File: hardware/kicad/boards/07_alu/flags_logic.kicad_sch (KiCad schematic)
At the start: 10 parts, among them U36 74HC86, U37 74LS08, U38 74LS540, U39 74LS377, U40 74LS377

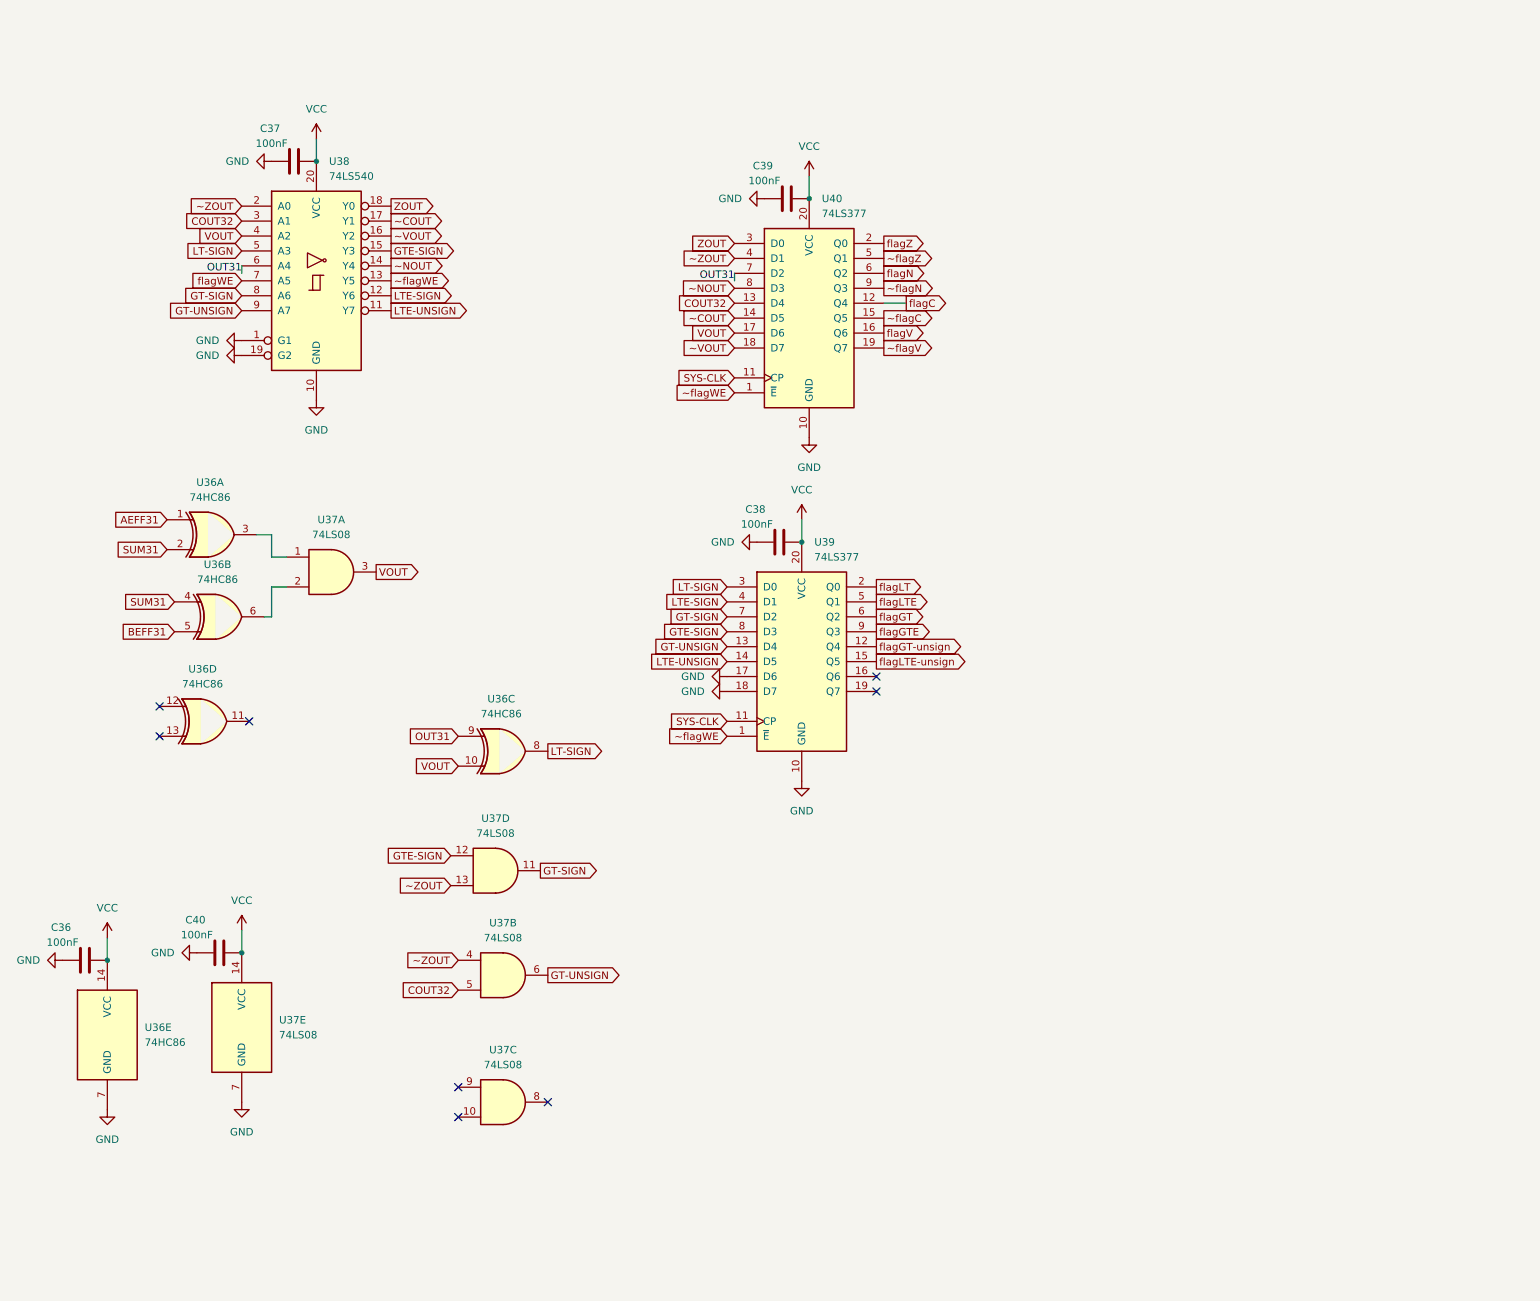
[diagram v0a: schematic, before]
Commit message: checkpoint: most recent 16b cell: ~120mm by 120mm
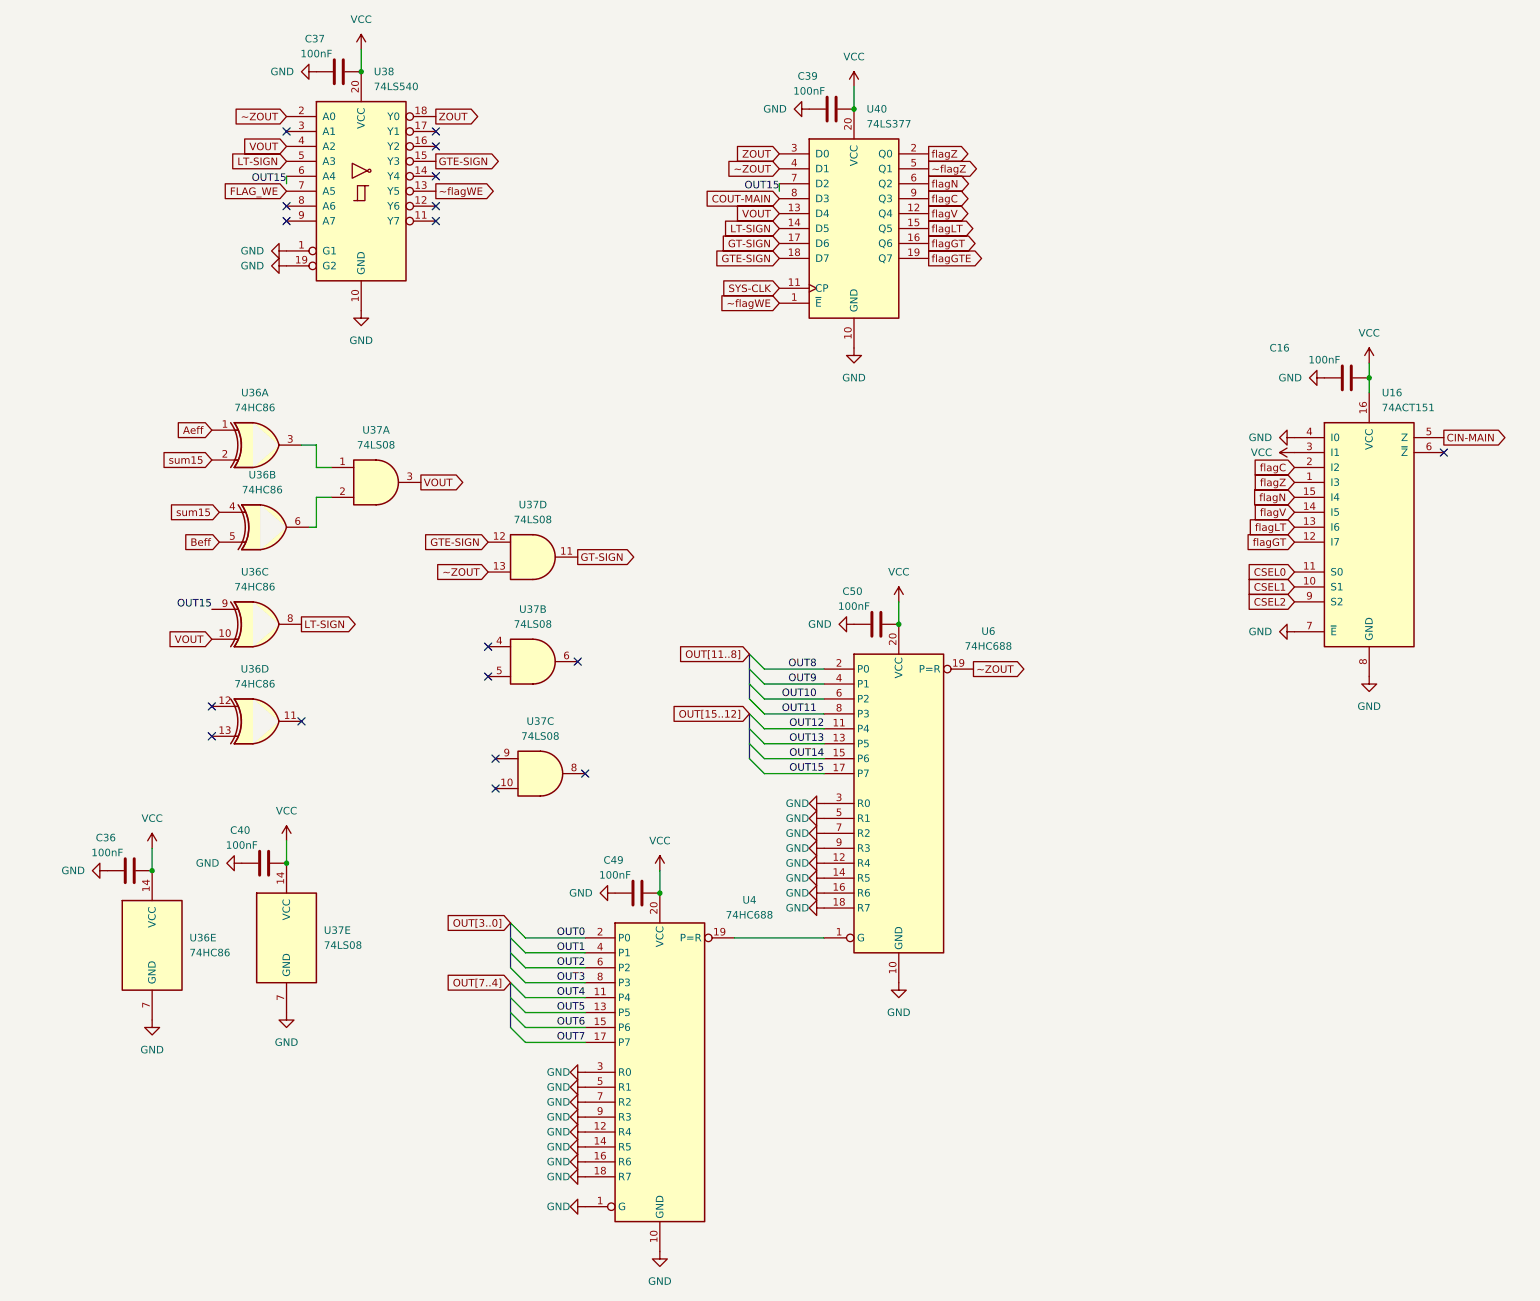
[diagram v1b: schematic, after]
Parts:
- removed C38: 100nF, Capacitor_SMD:C_0603_1608Metric, symbol Device:C
- removed U39: 74LS377, Package_SO:SOIC-20W_7.5x12.8mm_P1.27mm, symbol 74xx:74LS377
- added C16, C49, C50: 100nF, Capacitor_SMD:C_0603_1608Metric, symbol Device:C
- added U16: 74ACT151, Package_SO:SOIC-16_3.9x9.9mm_P1.27mm, symbol 74xx:74LS151
- added U4, U6: 74HC688, Package_SO:SOIC-20W_7.5x12.8mm_P1.27mm, symbol 74xx:74HC688
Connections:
- net ~flagC is gone; now on net flagLT: U40.15 (Q5)
- net ~flagN is gone; now on net flagC: U40.9 (Q3)
- net ~flagV is gone; now on net flagGTE: U40.19 (Q7)
- net GND: now also C16.1, C49.1, C50.1, U16.4 (I0), U16.7 (~{E}), U16.8 (GND), U4.1 (G), U4.10 (GND), U4.12 (R4), U4.14 (R5), U4.16 (R6), U4.18 (R7), U4.3 (R0), U4.5 (R1), U4.7 (R2), U4.9 (R3), U6.10 (GND), U6.12 (R4), U6.14 (R5), U6.16 (R6), U6.18 (R7), U6.3 (R0), U6.5 (R1), U6.7 (R2), U6.9 (R3)
- net GT-SIGN: now also U40.17 (D6); no longer U38.8 (A6)
- net GTE-SIGN: now also U40.18 (D7)
- net LT-SIGN: now also U40.14 (D5)
- net VCC: now also C16.2, C49.2, C50.2, U16.16 (VCC), U16.3 (I1), U4.20 (VCC), U6.20 (VCC)
- net VOUT: now also U40.13 (D4); no longer U40.17 (D6)
- net flagC: now also U16.2 (I2); no longer U40.12 (Q4)
- net flagGT: now also U40.16 (Q6), U16.12 (I7)
- net flagLT: now also U16.13 (I6)
- net flagN: now also U16.15 (I4)
- net flagV: now also U40.12 (Q4), U16.14 (I5); no longer U40.16 (Q6)
- net flagZ: now also U16.1 (I3)
- net ~ZOUT: now also U6.19 (P=R); no longer U37.4
- net AEFF31 renamed Aeff
- net BEFF31 renamed Beff
- removed net COUT32: U37.5, U38.3 (A1), U40.13 (D4)
- net GT-UNSIGN: no longer names the net of U38.9 (A7)
- net GT-UNSIGN: no longer U37.6
- net LTE-SIGN: no longer names the net of U38.12 (Y6)
- net LTE-UNSIGN: no longer names the net of U38.11 (Y7)
- net OUT31 renamed OUT15
- net OUT15: now also U6.17 (P7)
- net SUM31 renamed sum15
- net flagWE renamed FLAG_WE
- net ~COUT: no longer names the net of U38.17 (Y1)
- net ~COUT: no longer U40.14 (D5)
- net ~NOUT: no longer names the net of U38.14 (Y4)
- net ~NOUT: no longer U40.8 (D3)
- net ~VOUT: no longer names the net of U38.16 (Y2)
- net ~VOUT: no longer U40.18 (D7)
- new net: U4.19 (P=R), U6.1 (G)
- new net CIN-MAIN: U16.5 (Z)
- new net COUT-MAIN: U40.8 (D3)
- new net CSEL0: U16.11 (S0)
- new net CSEL1: U16.10 (S1)
- new net CSEL2: U16.9 (S2)
- new net OUT0: U4.2 (P0)
- new net OUT1: U4.4 (P1)
- new net OUT10: U6.6 (P2)
- new net OUT11: U6.8 (P3)
- new net OUT12: U6.11 (P4)
- new net OUT13: U6.13 (P5)
- new net OUT14: U6.15 (P6)
- new net OUT2: U4.6 (P2)
- new net OUT3: U4.8 (P3)
- new net OUT4: U4.11 (P4)
- new net OUT5: U4.13 (P5)
- new net OUT6: U4.15 (P6)
- new net OUT7: U4.17 (P7)
- new net OUT8: U6.2 (P0)
- new net OUT9: U6.4 (P1)
- no-connect marks 8 -> 18
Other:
- moved on the sheet: C36, C37, C39, C40, U36A, U36B, U36C, U36D, U36E, U37A, U37B, U37C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
